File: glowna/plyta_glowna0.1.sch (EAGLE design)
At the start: 136 parts, among them IC1 4504D, IC2 MAX481CSA, Q1 CSM-7X-DU, Q2 N-HEXFET-2D_SOT232-IRLL014N, Q3 N-HEXFET-2D_SOT232-IRLL014N, Q4 N-HEXFET-2D_SOT232-IRLL014N, Q5 N-HEXFET-2D_SOT232-IRLL014N, Q6 N-HEXFET-2D_SOT232-IRLL014N, X1 MINI-USB_SHIELD5P2-32005-601

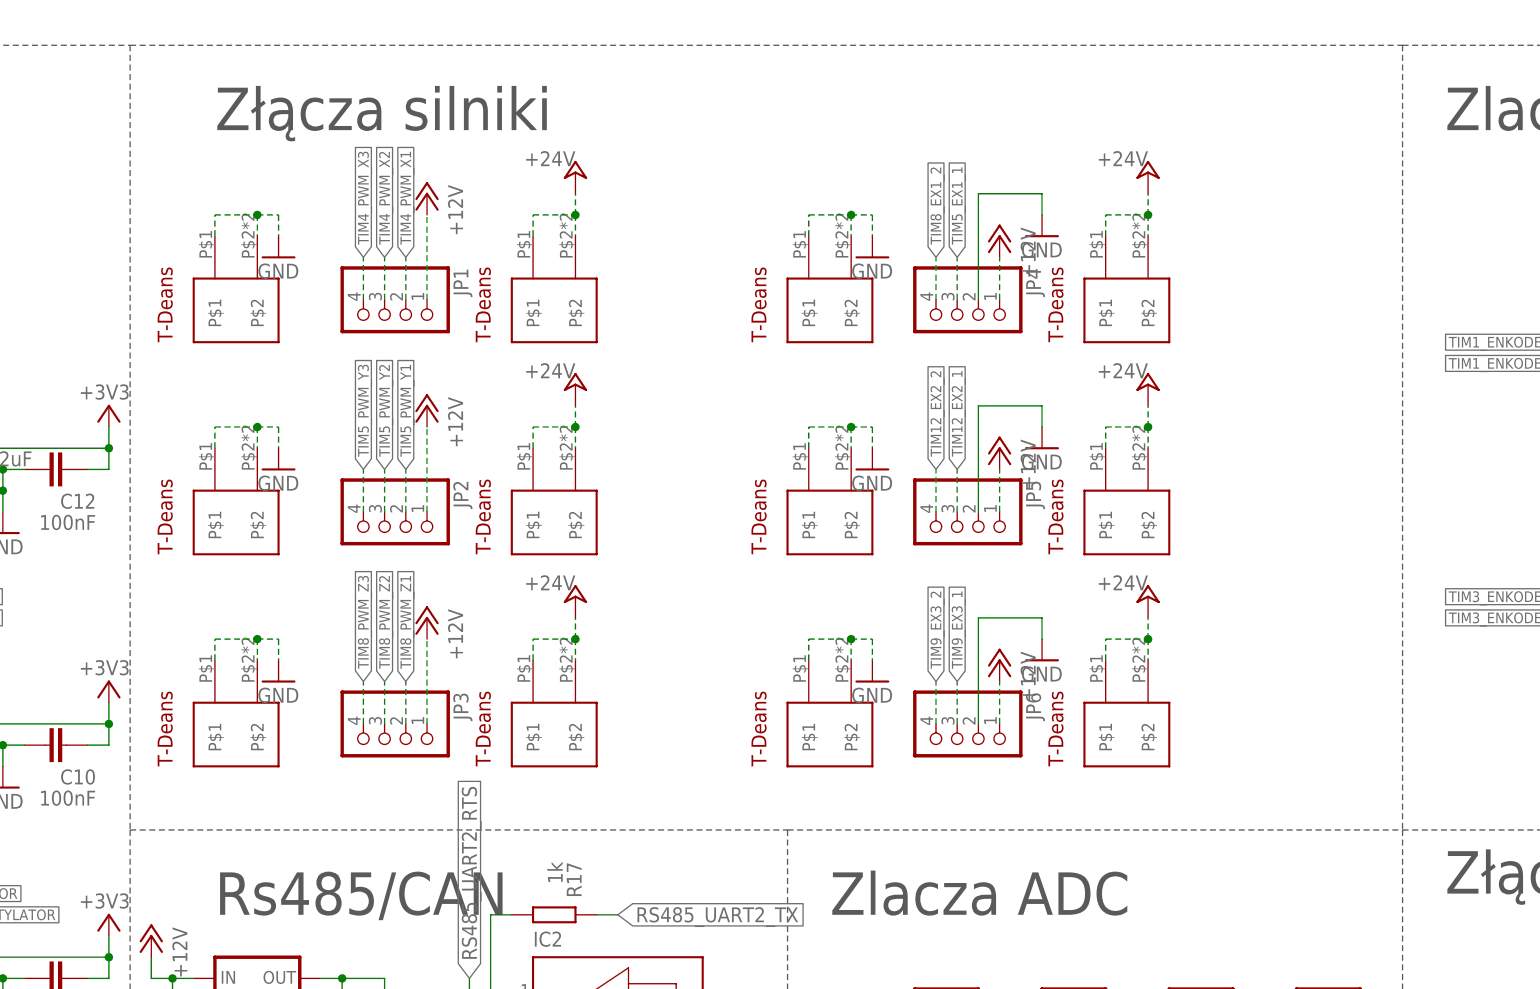
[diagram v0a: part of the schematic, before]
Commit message: zabezpieczenia
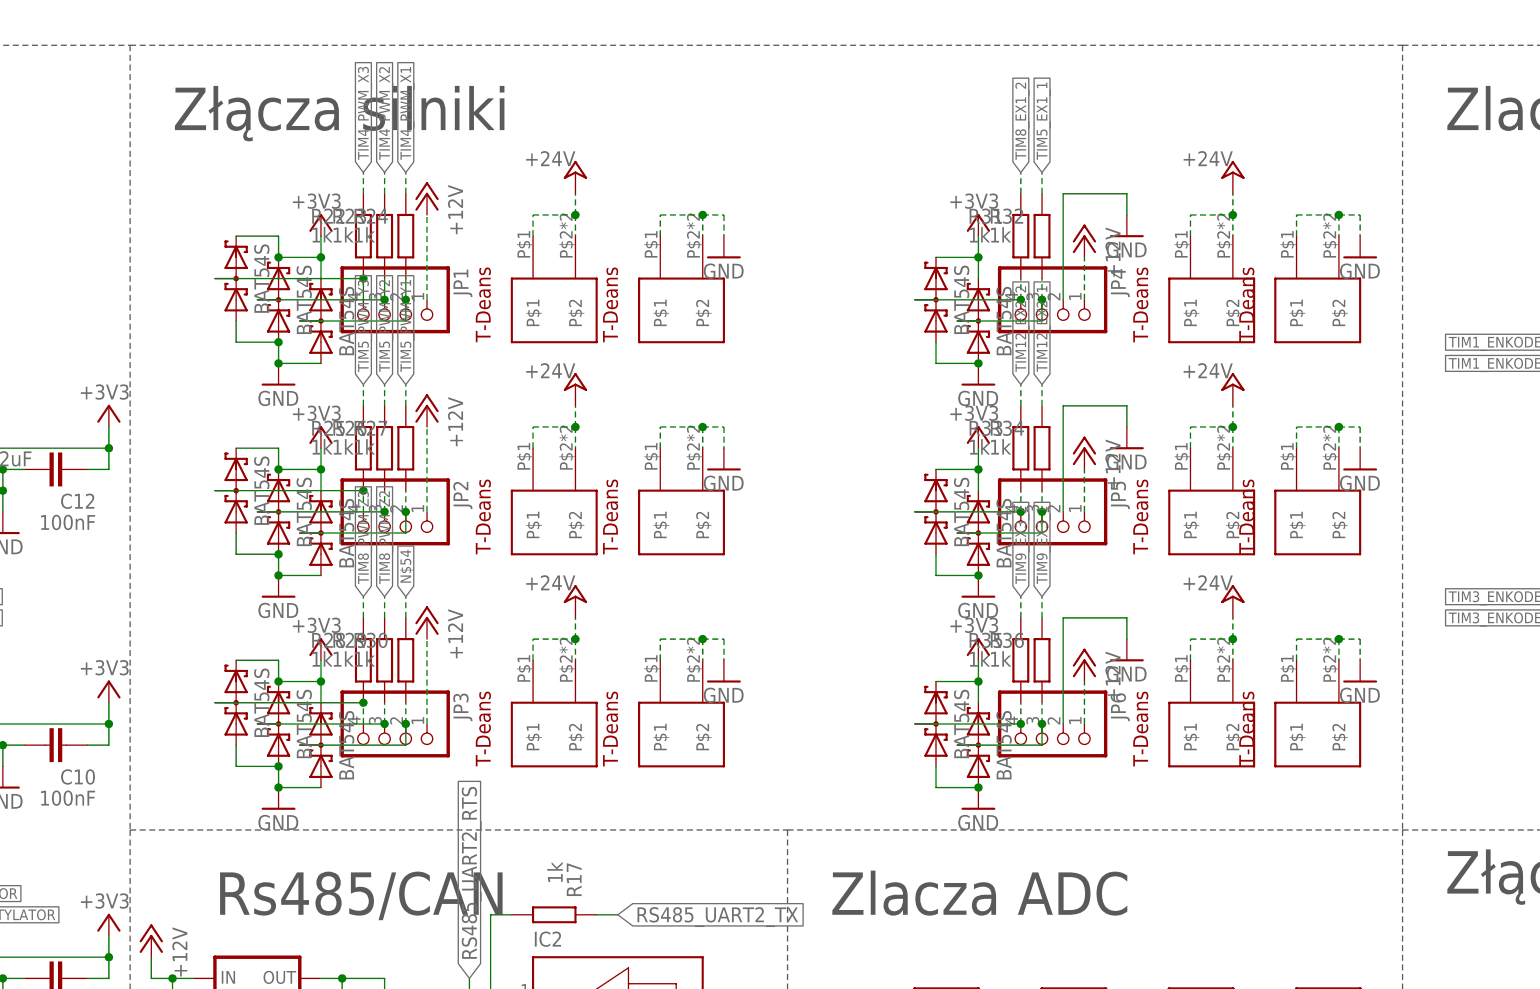
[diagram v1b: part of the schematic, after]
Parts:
- added D10, D11, D12, D13, D14, D15, D16, D17, D18, D19, D20, D5, D6, D7, D9: BAT54S, diode:BAT54S
- added R22, R23, R24, R25, R26, R27, R28, R29, R30, R31, R32, R33, R34, R35, R36: 1k, rcl:R-EU_R0603
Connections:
- new net N$41: D5.C1A2, JP1.4, R22.2
- new net N$45: D6.C1A2, JP1.3, R23.2
- new net N$46: D7.C1A2, JP1.2, R24.2
- new net N$48: D16.C1A2, JP4.4, R31.2
- new net N$49: D9.C1A2, JP2.4, R25.2
- new net N$50: D10.C1A2, JP2.3, R26.2
- new net N$51: D15.C1A2, JP4.3, R32.2
- new net N$52: D12.C1A2, JP3.4, R28.2
- new net N$53: D13.C1A2, JP3.3, R29.2
- new net N$54: R30.1
- new net N$55: D18.C1A2, JP5.4, R33.2
- new net N$56: D17.C1A2, JP5.3, R34.2
- new net N$57: D11.C1A2, JP2.2, R27.2
- new net N$58: D20.C1A2, JP6.4, R35.2
- new net N$59: D19.C1A2, JP6.3, R36.2
- net +3V3: now also D10.C2, D11.C2, D12.C2, D13.C2, D14.C2, D15.C2, D16.C2, D17.C2, D18.C2, D19.C2, D20.C2, D5.C2, D6.C2, D7.C2, D9.C2
- net GND: now also D10.A1, D11.A1, D12.A1, D13.A1, D14.A1, D15.A1, D16.A1, D17.A1, D18.A1, D19.A1, D20.A1, D5.A1, D6.A1, D7.A1, D9.A1
- net TIM12_EX2_1: now also R34.1; no longer JP5.3
- net TIM12_EX2_2: now also R33.1; no longer JP5.4
- net TIM4_PWM_X1: now also R24.1; no longer JP1.2
- net TIM4_PWM_X2: now also R23.1; no longer JP1.3
- net TIM4_PWM_X3: now also R22.1; no longer JP1.4
- net TIM5_EX1_1: now also R32.1; no longer JP4.3
- net TIM5_PWM_Y1: now also R27.1; no longer JP2.2
- net TIM5_PWM_Y2: now also R26.1; no longer JP2.3
- net TIM5_PWM_Y3: now also R25.1; no longer JP2.4
- net TIM8_EX1_2: now also R31.1; no longer JP4.4
- net TIM8_PWM_Z1: now also D14.C1A2, R30.2
- net TIM8_PWM_Z2: now also R29.1; no longer JP3.3
- net TIM8_PWM_Z3: now also R28.1; no longer JP3.4
- net TIM9_EX3_1: now also R36.1; no longer JP6.3
- net TIM9_EX3_2: now also R35.1; no longer JP6.4
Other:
- moved on the sheet: JP4, JP5, JP6
